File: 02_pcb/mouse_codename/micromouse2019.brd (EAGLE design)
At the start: 45 x 50 mm, 78 parts

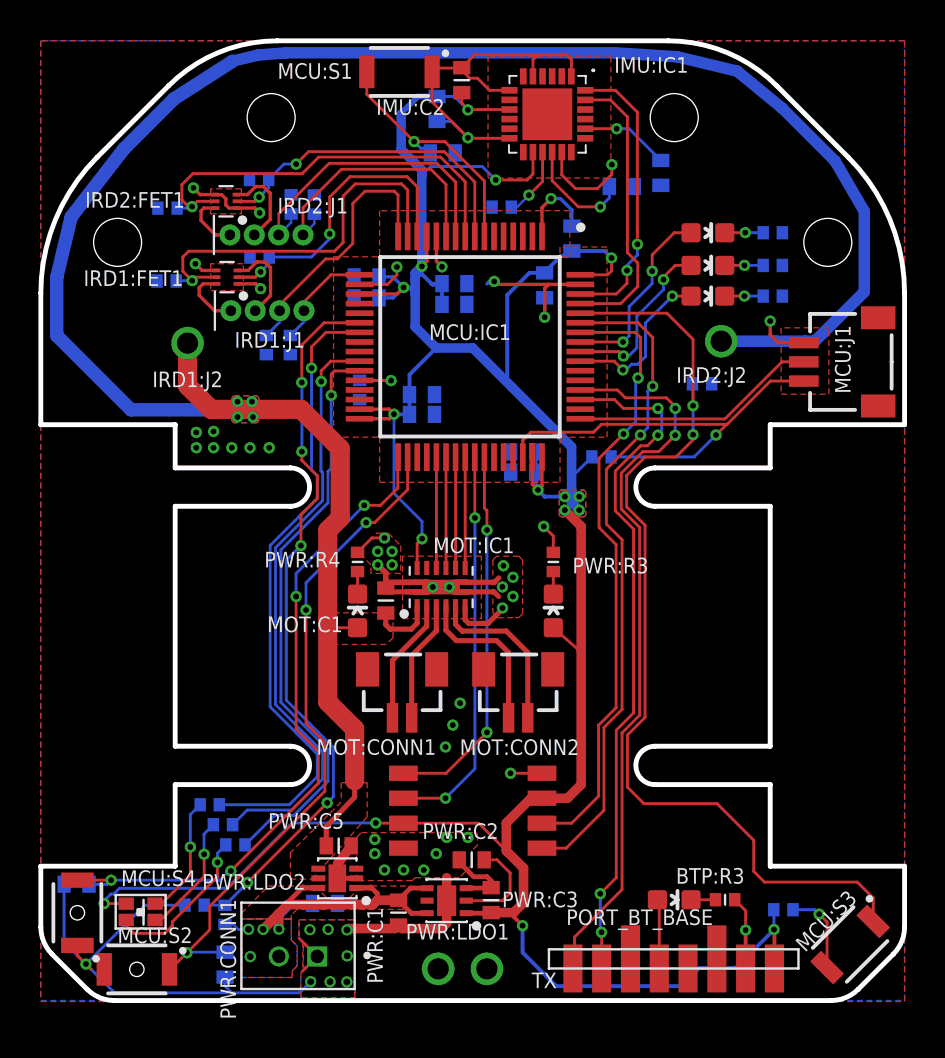
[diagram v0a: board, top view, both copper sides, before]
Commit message: drc rule check ok
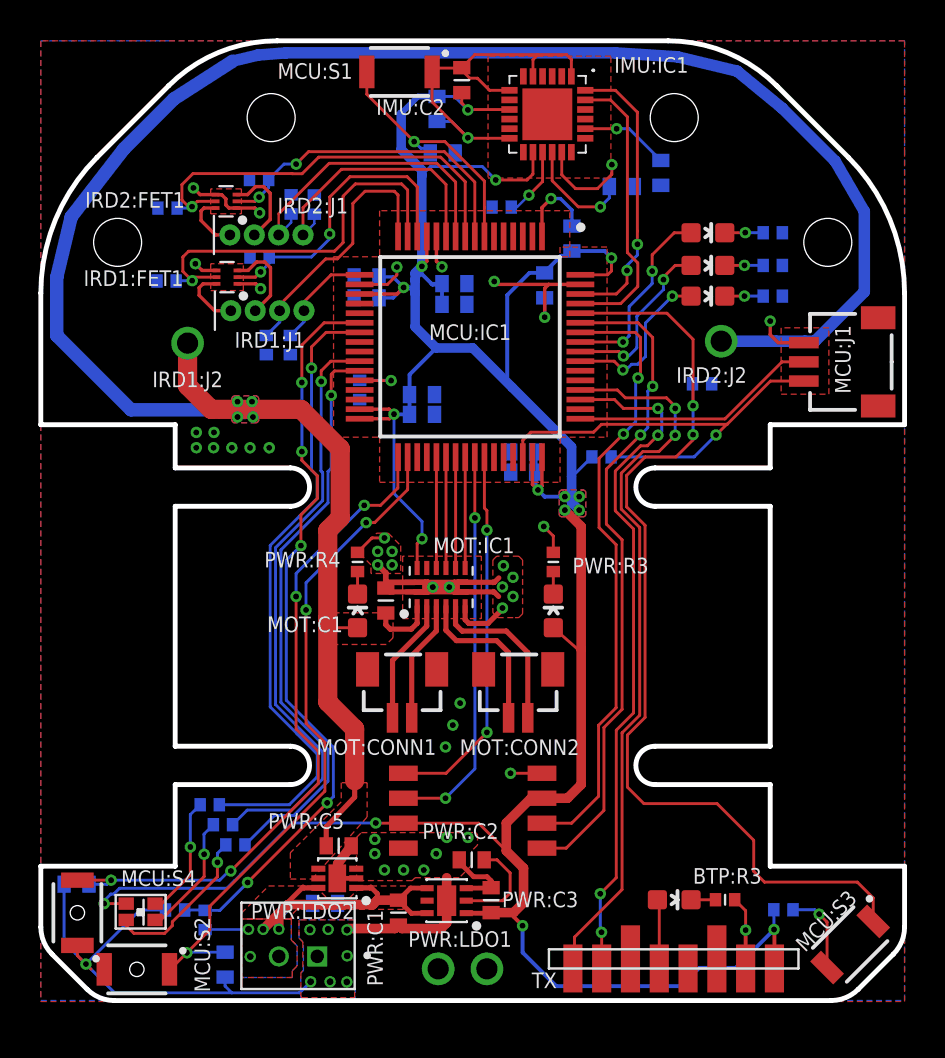
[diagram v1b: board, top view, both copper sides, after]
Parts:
- MCU:R1, MCU:R10: device rcl:R0402 -> 0-micromouse2019:R0402
- moved PWR:R1 1.06 mm to (8.56, 4.20)
- moved PWR:R2 1.05 mm to (6.99, 4.72)
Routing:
- net GND: track 123.5 -> 119.5 mm
- net V_BAT_LEVEL: track 38.1 -> 39.3 mm
- net PWR:V_BAT_IN: track 19.7 -> 20.6 mm
